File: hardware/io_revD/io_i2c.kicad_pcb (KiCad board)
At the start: 2 copper layers, 85.7 x 76.8 mm, 37 parts, among them J1 Target Interface, 2716 Pinout, J2 Jumper Block, J3 Jumper Block, J4 Target Interface, 2716 Pinout, Q1 2N7000, U1 2716, U2 74HCT74, U3 74HCT125, U4 74HCT138, U5 74LS04, U6 MCP23018-E_SP, U7 74HCT138

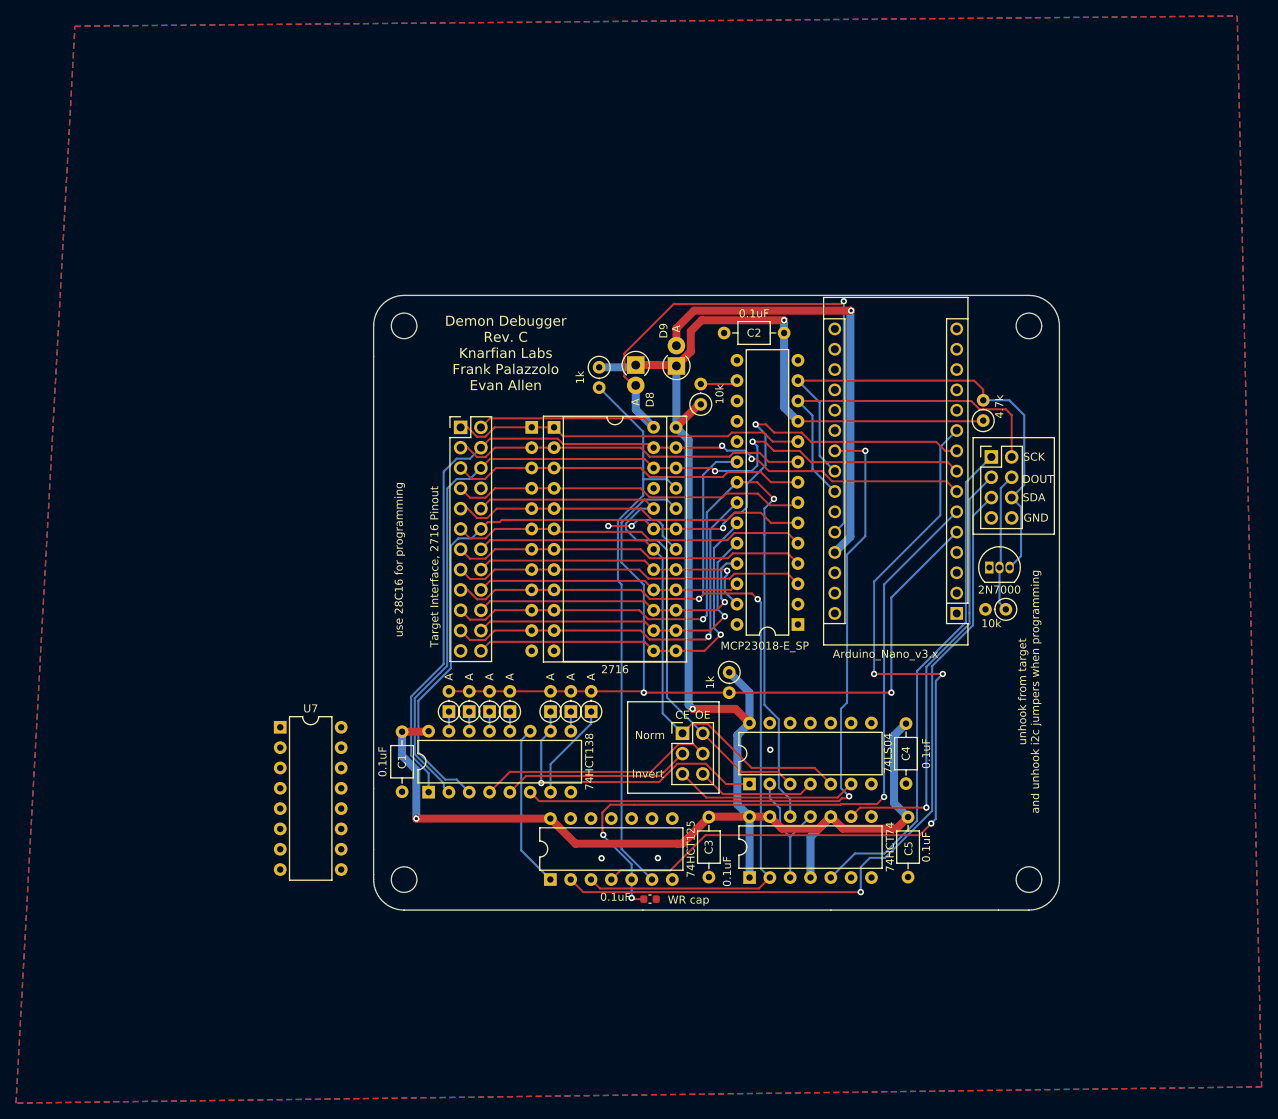
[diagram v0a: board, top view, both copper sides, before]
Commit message: revD board
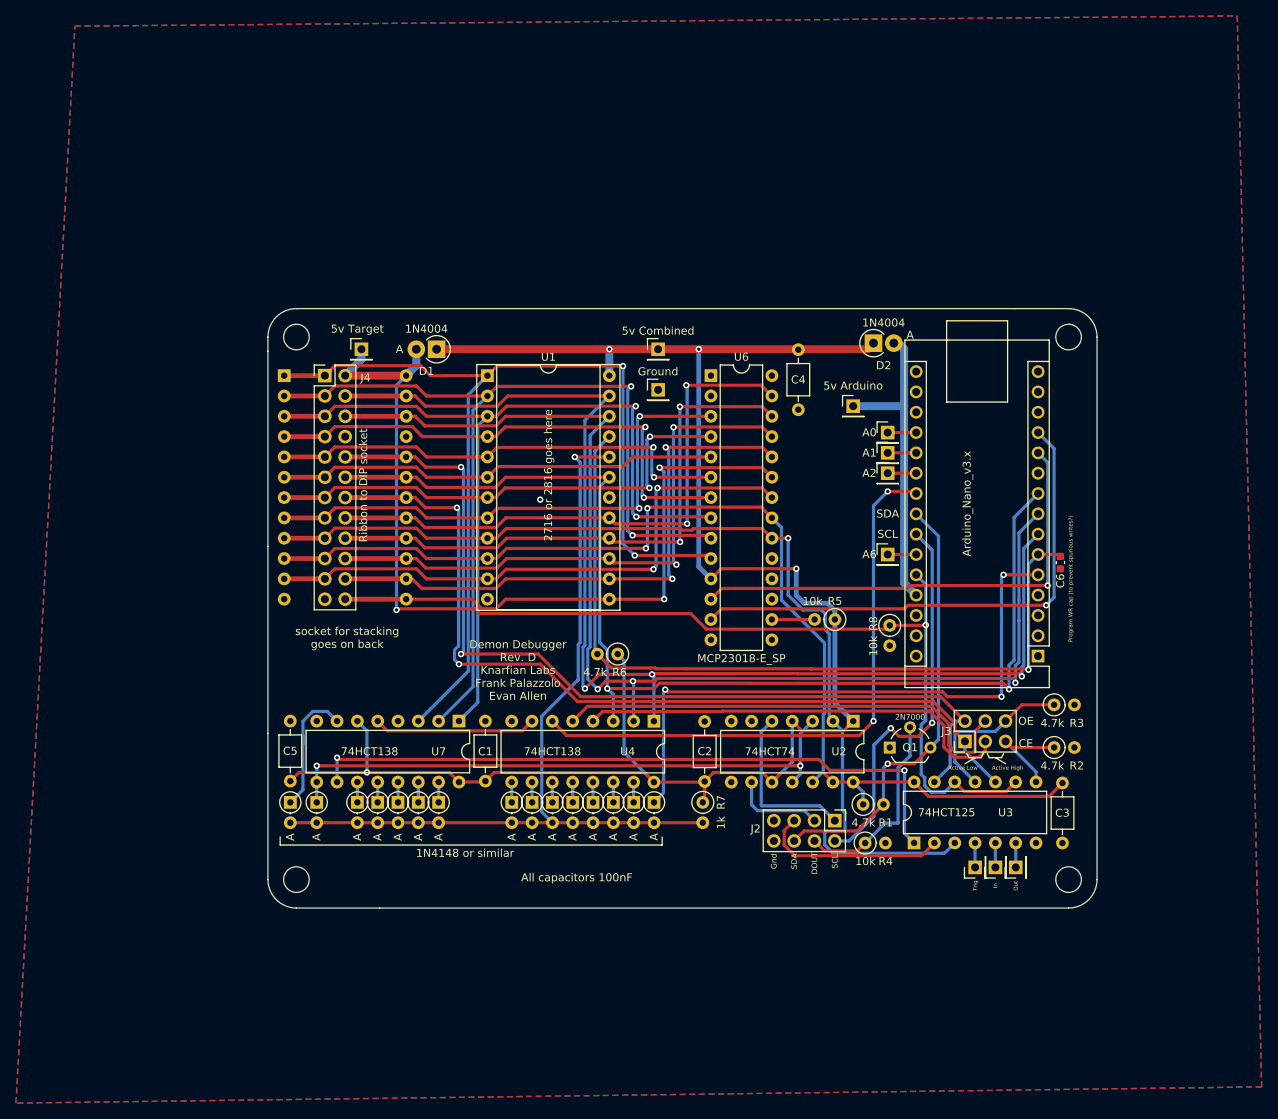
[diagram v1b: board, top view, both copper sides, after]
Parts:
- removed the REF** at (101.6, 95.9)
- removed the REF** at (179.7, 95.9)
- removed the REF** at (101.6, 165.1)
- removed the REF** at (179.7, 165.1)
- removed U5: 74LS04, Package_DIP:DIP-14_W7.62mm
- added D10: 1N4148, Diode_THT:D_DO-35_SOD27_P2.54mm_Vertical_AnodeUp, F.Cu at (115.1, 155.4)
- added D11: 1N4148, Diode_THT:D_DO-35_SOD27_P2.54mm_Vertical_AnodeUp, F.Cu at (105.9, 155.4)
- added D12: 1N4148, Diode_THT:D_DO-35_SOD27_P2.54mm_Vertical_AnodeUp, F.Cu at (103.4, 155.4)
- added D13: 1N4148, Diode_THT:D_DO-35_SOD27_P2.54mm_Vertical_AnodeUp, F.Cu at (100.8, 155.4)
- added D14: 1N4148, Diode_THT:D_DO-35_SOD27_P2.54mm_Vertical_AnodeUp, F.Cu at (98.3, 155.4)
- added D15: 1N4148, Diode_THT:D_DO-35_SOD27_P2.54mm_Vertical_AnodeUp, F.Cu at (95.8, 155.4)
- added D16: 1N4148, Diode_THT:D_DO-35_SOD27_P2.54mm_Vertical_AnodeUp, F.Cu at (90.7, 155.4)
- added D17: 1N4148, Diode_THT:D_DO-35_SOD27_P2.54mm_Vertical_AnodeUp, F.Cu at (87.4, 155.4)
- added J10: Conn_01x01, Connector_PinHeader_2.54mm:PinHeader_1x01_P2.54mm_Vertical, F.Cu at (162.1, 114.3)
- added J11: Conn_01x01, Connector_PinHeader_2.54mm:PinHeader_1x01_P2.54mm_Vertical, F.Cu at (162.1, 124.5)
- added J12: Conn_01x01, Connector_PinHeader_2.54mm:PinHeader_1x01_P2.54mm_Vertical, F.Cu at (96.3, 98.8)
- added J13: Conn_01x01, Connector_PinHeader_2.54mm:PinHeader_1x01_P2.54mm_Vertical, F.Cu at (133.3, 98.8)
- added J14: Conn_01x01, Connector_PinHeader_2.54mm:PinHeader_1x01_P2.54mm_Vertical, F.Cu at (133.3, 103.9)
- added J15: Conn_01x01, Connector_PinHeader_2.54mm:PinHeader_1x01_P2.54mm_Vertical, F.Cu at (157.7, 105.9)
- added J5: Conn_01x01, Connector_PinHeader_2.54mm:PinHeader_1x01_P2.54mm_Vertical, F.Cu at (175.5, 163.6)
- added J6: Conn_01x01, Connector_PinHeader_2.54mm:PinHeader_1x01_P2.54mm_Vertical, F.Cu at (173.0, 163.6)
- added J7: Conn_01x01, Connector_PinHeader_2.54mm:PinHeader_1x01_P2.54mm_Vertical, F.Cu at (178.1, 163.6)
- added J8: Conn_01x01, Connector_PinHeader_2.54mm:PinHeader_1x01_P2.54mm_Vertical, F.Cu at (162.1, 109.2)
- added J9: Conn_01x01, Connector_PinHeader_2.54mm:PinHeader_1x01_P2.54mm_Vertical, F.Cu at (162.1, 111.8)
- added R6: 4.7k, Resistor_THT:R_Axial_DIN0207_L6.3mm_D2.5mm_P2.54mm_Vertical, F.Cu at (128.3, 136.9)
- added R7: 1k, Resistor_THT:R_Axial_DIN0207_L6.3mm_D2.5mm_P2.54mm_Vertical, F.Cu at (138.9, 155.4)
- added R8: 10k, Resistor_THT:R_Axial_DIN0207_L6.3mm_D2.5mm_P2.54mm_Vertical, F.Cu at (162.3, 133.3)
- added REF**: MountingHole_3.2mm_M3, MountingHole:MountingHole_3.2mm_M3, F.Cu at (184.7, 97.3)
- added REF**: MountingHole_3.2mm_M3, MountingHole:MountingHole_3.2mm_M3, F.Cu at (88.1, 97.3)
- added REF**: MountingHole_3.2mm_M3, MountingHole:MountingHole_3.2mm_M3, F.Cu at (88.1, 165.1)
- added REF**: MountingHole_3.2mm_M3, MountingHole:MountingHole_3.2mm_M3, F.Cu at (184.7, 165.1)
- D1, D2: value 1N4148 -> 1N4004; footprint Diode_THT:D_DO-35_SOD27_P2.54mm_Vertical_AnodeUp -> Diode_THT:D_DO-41_SOD81_P2.54mm_Vertical_AnodeUp
- D8, D9: value 1N4004 -> 1N4148; footprint Diode_THT:D_DO-41_SOD81_P2.54mm_Vertical_AnodeUp -> Diode_THT:D_DO-35_SOD27_P2.54mm_Vertical_AnodeUp
- Q1: footprint Package_TO_SOT_THT:TO-92_Inline -> Package_TO_SOT_THT:TO-92_Wide
- R2, R3: value 1k -> 4.7k
- moved C5 77.3 mm to (87.4, 152.8), turned to 90 degrees
- moved R3 70.8 mm to (182.9, 143.3), turned to 0 degrees
- moved D2 68.4 mm to (160.3, 98.0), turned to 0 degrees
- moved C6 66.3 mm to (183.6, 125.5), turned to -90 degrees
- moved D9 57.5 mm to (117.6, 155.4), turned to -90 degrees
- moved C2 56.9 mm to (139.2, 152.8), turned to 90 degrees
- moved D8 55.6 mm to (120.1, 155.4)
- moved R1 50.3 mm to (159.0, 155.7), turned to 0 degrees
- moved J2 49.5 mm to (155.4, 157.7), turned to -90 degrees
- moved C4 48.6 mm to (150.9, 98.9)
- moved U3 45.7 mm to (165.3, 160.5)
- moved D1 45.3 mm to (105.7, 98.8), turned to 180 degrees
- moved C3 44.4 mm to (183.9, 153.0)
- moved R2 41.7 mm to (182.9, 148.6), turned to 0 degrees
- moved J3 35.3 mm to (171.7, 147.8), turned to 90 degrees
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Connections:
- A1 pad 10: /WR enable -> unconnected-(A1-Pad10)
- A1 pad 11: unconnected-(A1-Pad11) -> /SCL2
- A1 pad 12: unconnected-(A1-Pad12) -> /SDA2
- A1 pad 19: unconnected-(A1-Pad19) -> Net-(A1-Pad19)
- A1 pad 20: unconnected-(A1-Pad20) -> Net-(A1-Pad20)
- A1 pad 21: unconnected-(A1-Pad21) -> Net-(A1-Pad21)
- A1 pad 25: unconnected-(A1-Pad25) -> Net-(A1-Pad25)
- D1 pad 1: Net-(D1-Pad1) -> +5V
- D1 pad 2: /program OE -> +5VD
- D2 pad 1: Net-(D2-Pad1) -> +5V
- D2 pad 2: /program OE -> +5VA
- D3 pad 1: Net-(D3-Pad1) -> /program OE
- D3 pad 2: /program OE -> Net-(D10-Pad2)
- D4 pad 2: /program OE -> Net-(D10-Pad2)
- D5 pad 2: /program OE -> Net-(D10-Pad2)
- D6 pad 2: /program OE -> Net-(D10-Pad2)
- D7 pad 2: /program OE -> Net-(D10-Pad2)
- D8 pad 1: +5V -> Net-(D8-Pad1)
- D8 pad 2: +5VD -> Net-(D10-Pad2)
- D9 pad 1: +5V -> Net-(D9-Pad1)
- D9 pad 2: +5VA -> Net-(D10-Pad2)
- R2 pad 1: +5V -> Net-(J3-Pad5)
- R2 pad 2: /program OE -> GND
- R3 pad 1: +5V -> Net-(J3-Pad6)
- R3 pad 2: Net-(R3-Pad2) -> GND
- U1 pad 20: /program OE -> Net-(D10-Pad2)
- U1 pad 21: Net-(R3-Pad2) -> /program WR
- U2 pad 11: Net-(U2-Pad11) -> Net-(D16-Pad1)
- U2 pad 3: Net-(U2-Pad11) -> Net-(D16-Pad1)
- U3 pad 10: GND -> /Target CE
- U3 pad 11: unconnected-(U3-Pad11) -> Net-(J3-Pad6)
- U3 pad 12: GND -> +5VD
- U3 pad 13: GND -> /Target OE
- U3 pad 4: /WR enable -> Net-(J6-Pad1)
- U3 pad 5: /program WR -> Net-(J5-Pad1)
- U3 pad 6: Net-(R3-Pad2) -> Net-(J7-Pad1)
- U3 pad 8: unconnected-(U3-Pad8) -> Net-(J3-Pad5)
- U3 pad 9: GND -> +5VD
- U4 pad 10: Net-(D5-Pad1) -> Net-(D9-Pad1)
- U4 pad 11: Net-(U3-Pad1) -> Net-(D8-Pad1)
- U4 pad 12: Net-(D4-Pad1) -> Net-(D7-Pad1)
- U4 pad 13: Net-(D3-Pad1) -> Net-(D6-Pad1)
- U4 pad 14: Net-(D2-Pad1) -> Net-(D5-Pad1)
- U4 pad 15: Net-(D1-Pad1) -> Net-(D4-Pad1)
- U4 pad 4: Net-(J3-Pad4) -> Net-(J3-Pad3)
- U4 pad 5: Net-(J3-Pad3) -> Net-(J3-Pad4)
- U4 pad 7: Net-(D7-Pad1) -> Net-(U4-Pad7)
- U4 pad 9: Net-(D6-Pad1) -> Net-(D10-Pad1)
- U7 pad 1: unconnected-(U7-Pad1) -> /A5
- U7 pad 10: unconnected-(U7-Pad10) -> Net-(U3-Pad1)
- U7 pad 11: unconnected-(U7-Pad11) -> Net-(D15-Pad1)
- U7 pad 12: unconnected-(U7-Pad12) -> Net-(D14-Pad1)
- U7 pad 13: unconnected-(U7-Pad13) -> Net-(D13-Pad1)
- U7 pad 14: unconnected-(U7-Pad14) -> Net-(D12-Pad1)
- U7 pad 15: unconnected-(U7-Pad15) -> Net-(D11-Pad1)
- U7 pad 16: unconnected-(U7-Pad16) -> +5V
- U7 pad 2: unconnected-(U7-Pad2) -> /A6
- U7 pad 3: unconnected-(U7-Pad3) -> /A7
- U7 pad 4: unconnected-(U7-Pad4) -> GND
- U7 pad 5: unconnected-(U7-Pad5) -> Net-(U4-Pad7)
- U7 pad 6: unconnected-(U7-Pad6) -> +5V
- U7 pad 7: unconnected-(U7-Pad7) -> Net-(D17-Pad1)
- U7 pad 8: unconnected-(U7-Pad8) -> GND
- U7 pad 9: unconnected-(U7-Pad9) -> Net-(D16-Pad1)
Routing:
- net /WR enable: track 105.5 -> 0.00 mm, vias 3 -> 0
- net Net-(D10-Pad2): track 0.00 -> 104.4 mm, vias 0 -> 1
- net /A7: track 44.3 -> 124.6 mm, vias 0 -> 2
- net Net-(D16-Pad1): track 0.00 -> 73.7 mm, vias 0 -> 2
- net /A6: track 44.3 -> 117.1 mm, vias 0 -> 2
- net Net-(R3-Pad2): track 71.4 -> 0.00 mm
- net Net-(J2-Pad5): track 94.1 -> 23.6 mm, vias 1 -> 0
- net /SDA2: track 0.00 -> 65.5 mm, vias 0 -> 1
- net /A5: track 44.5 -> 109.3 mm, vias 0 -> 2
- net Net-(U3-Pad1): track 20.5 -> 84.2 mm, vias 0 -> 2
- net +5VD: track 92.9 -> 153.4 mm, vias 1 -> 2
- net /SCL2: track 0.00 -> 59.9 mm, vias 0 -> 1
- net Net-(J2-Pad3): track 54.5 -> 11.5 mm, vias 1 -> 0
- net /Target OE: track 72.0 -> 115.0 mm, vias 0 -> 2
- net Net-(J2-Pad1): track 63.0 -> 21.1 mm
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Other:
- board size 85.7 x 76.8 mm -> 103.6 x 74.9 mm
- board text added: "1"
- board text added: "1N4148 or similar"
- board text added: "2716 or 2816 goes here"
- board text added: "5v Arduino"
- board text added: "5v Combined"
- board text added: "5v Target"
- board text added: "A0"
- board text added: "A1"
- board text added: "A2"
- board text added: "A6"
- board text added: "Active High"
- board text added: "Active Low"
- board text added: "All capacitors 100nF"
- board text added: "Demon Debugger Rev. D Knarfian Labs Frank Palazzolo Evan Allen"
- board text added: "Disconnect target and J2 jumpers for programming"
- board text added: "Gnd"
- board text added: "Ground"
- board text added: "In"
- board text added: "Jumper across all J2 pads for ROM-mapped I/O"
- board text added: "Minimal interface is the arduino, Q1, R4, and R5 connected out J2"
- board text added: "Out"
- board text added: "Program WR cap (to prevent spurious writes?)"
- board text added: "Ribbon to DIP socket"
- board text added: "SCL"
- board text added: "Trig"
- board text added: "U6, C4, and U1 being a 2816 enables onboard reprogramming of the flash chip"
- board text added: "socket for stacking goes on back"
- board text removed: "Demon Debugger Rev. C Knarfian Labs Frank Palazzolo Evan Allen"
- board text removed: "GND"
- board text removed: "Invert"
- board text removed: "Norm"
- board text removed: "SCK"
- board text removed: "WR cap"
- board text removed: "unhook from target and unhook i2c jumpers when programming"
- board text removed: "use 28C16 for programming"
